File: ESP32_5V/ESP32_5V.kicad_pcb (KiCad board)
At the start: 4 copper layers, 90 x 70 mm, 92 parts, among them J1 Barrel_Jack_MountingPin, J10 Conn_01x11, J11 Conn_01x11, J12 Conn_01x11, J13 Conn_01x11, J15 Screw_Terminal_01x11, J16 Screw_Terminal_01x11, J2 Conn_01x11, J3 Conn_01x11, J4 Conn_01x11, J5 Conn_01x11, J6 Conn_01x11, J7 Conn_01x11, J8 Conn_01x11, J9 Conn_01x11, U1 TPS563201, U2 TPS563201, U3 SN74LVC245APW, U4 SN74LVC245APW, U5 SN74LVC245APW

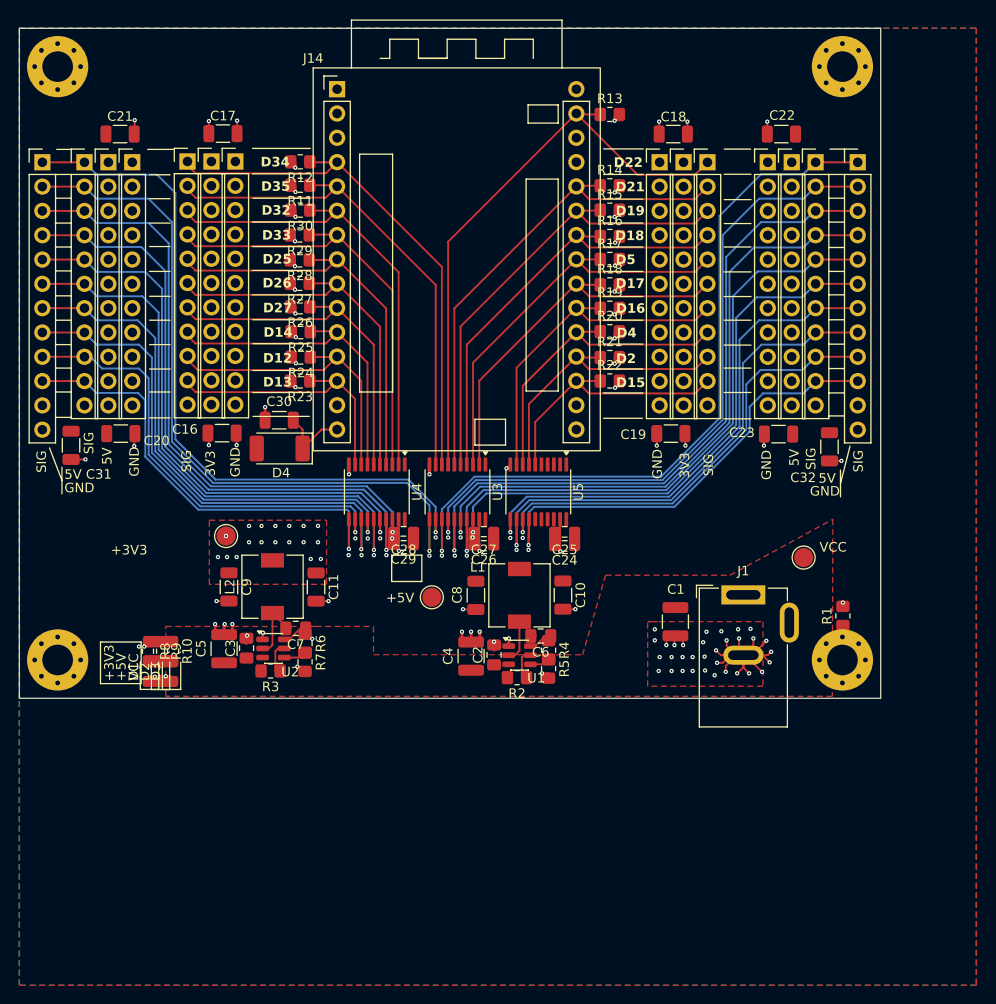
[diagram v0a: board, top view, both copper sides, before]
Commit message: update
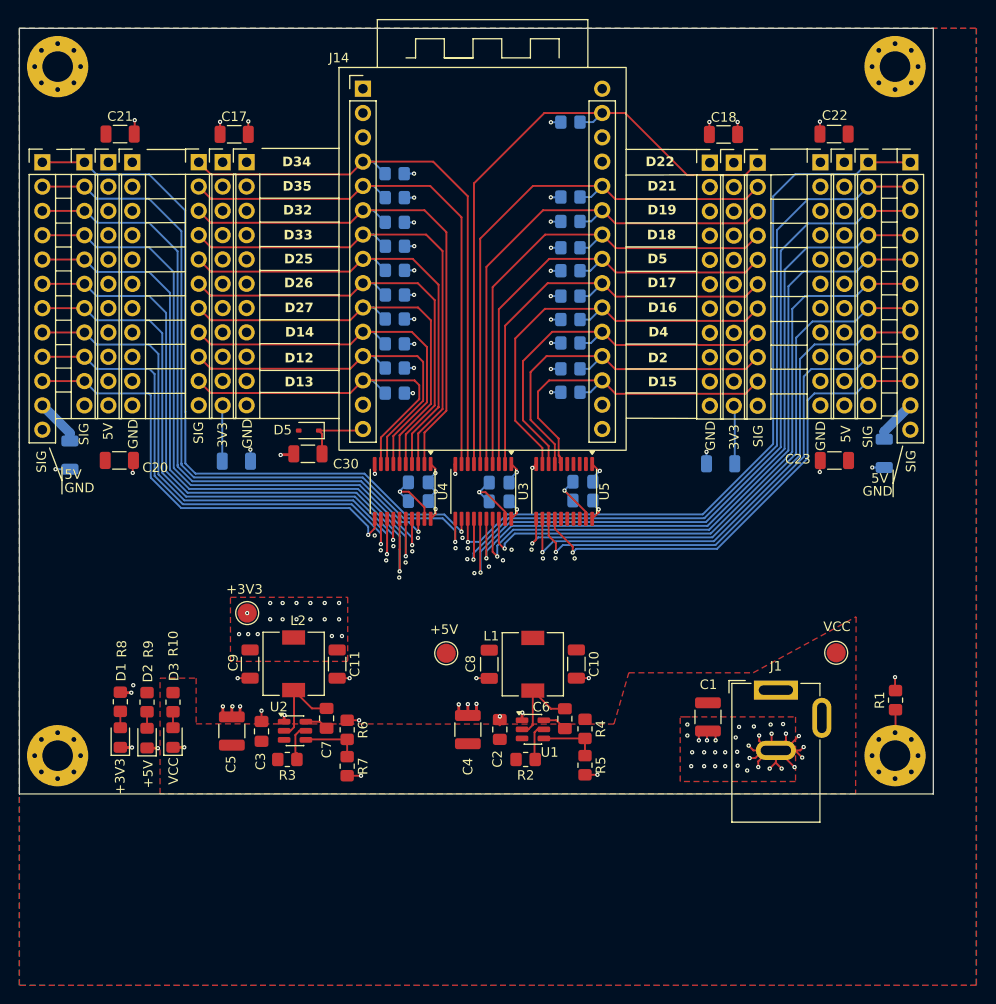
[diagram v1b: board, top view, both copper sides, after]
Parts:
- removed D4: 1N5712UR, Diode_SMD:D_MELF
- added D5: 1N5819WS, Diode_SMD:D_SOD-323, F.Cu at (123.8, 85.4)
- C16, C19, C24, C25, C26, C27, C28, C29, C31, C32, R11, R12, R13, R14, R15, R16, R17, R18, R19, R20, R21, R22, R23, R24, R25, R26, R27, R28, R29, R30: moved to B.Cu
- moved R7 11.8 mm to (127.8, 120.5)
- moved H3 11.4 mm to (185.1, 119.4)
- moved R5 10.8 mm to (152.7, 120.4)
- moved J1 10.5 mm to (172.7, 112.5)
- moved TP1 10.5 mm to (178.9, 108.7)
- moved C1 10.5 mm to (165.6, 115.3)
- moved R1 10.4 mm to (185.2, 113.6)
- moved R6 10.0 mm to (127.8, 116.7)
- moved R27 10.0 mm to (132.8, 71.3), turned to 0 degrees
- moved R29 10.0 mm to (132.8, 66.2), turned to 0 degrees
- moved H4 10.0 mm to (97.6, 119.4)
- moved R28 10.00 mm to (132.8, 68.7), turned to 0 degrees
- moved R11 9.96 mm to (132.8, 61.1), turned to 0 degrees
- moved R23 9.96 mm to (132.8, 81.5), turned to 0 degrees
- moved R26 9.96 mm to (132.8, 73.8), turned to 0 degrees
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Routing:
- net +5V: track 0.00 -> 26.9 mm, vias 0 -> 7
- net GND: track 102.2 -> 121.4 mm, vias 110 -> 111
- net +3V3: track 7.19 -> 17.0 mm, vias 24 -> 22
- net /Conector_3V3/D16: track 36.7 -> 45.6 mm
- net /Conector_3V3/D2: track 31.1 -> 39.0 mm
- net /Conector_5V/D21_5V: track 71.9 -> 79.7 mm
- net /Conector_3V3/D15: track 28.3 -> 36.0 mm
- net /Conector_3V3/D4: track 33.9 -> 41.6 mm
- net /Conector_3V3/D13: track 29.8 -> 37.1 mm
- net /Conector_5V/D18_5V: track 66.5 -> 73.8 mm
- net /Conector_5V/D25_5V: track 59.5 -> 66.8 mm
- net /Conector_3V3/D12: track 32.7 -> 39.9 mm
- net /Conector_5V/D26_5V: track 60.1 -> 67.1 mm
- net /Conector_3V3/D27: track 38.2 -> 45.1 mm
- net /Conector_3V3/D33: track 46.7 -> 53.4 mm
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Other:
- board size 90 x 70 mm -> 95.5 x 80 mm
